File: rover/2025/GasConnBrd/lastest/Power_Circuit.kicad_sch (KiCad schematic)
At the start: 0 parts

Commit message: PCB finit
A faire approuver au besoin
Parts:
- added C18, C19, C24, C25: 10uF, Capacitor_SMD:C_0805_2012Metric_Pad1.18x1.45mm_HandSolder, symbol RoverLibrary:C_0805
- added D4: CVJ10F30, RoverFootprint:Diode_schottky-CVJ10F30, symbol RoverLibrary:Diode_Schottchy_CVJ10F30
- added J3, J6: Eth-Horiz, RoverFootprint:Ethernet_Horizontal, symbol RoverLibrary:Eth-Horiz-54601-908WPLF
- added TP6, TP7: TestPoint, TestPoint:TestPoint_Plated_Hole_D2.0mm, symbol RoverLibrary:TestPoint
- added U1: R-78E5.0-0.5, Converter_DCDC:Converter_DCDC_RECOM_R-78E-0.5_THT, symbol Regulator_Switching:R-78E5.0-0.5
- added U7: LDO-TLV74033PDBVR, Package_TO_SOT_SMD:SOT-23-5_HandSoldering, symbol RoverLibrary:LDO-TLV74033PDBVR
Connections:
- new net +24V: C19.1, J3.5, J3.7, J6.5, J6.7, U1.1 (IN)
- new net +3.3V: C24.1, TP6.1, U7.5 (OUTPUT)
- new net +5V: C18.1, D4.4, D4.5, TP7.1, U7.1 (INPUT), U7.3 (EN)
- new net +5V_ETH: C25.1, D4.3, U1.3 (OUT)
- new net +5V_USB: D4.1
- new net CAN_N: J3.2 (CANL), J6.3
- new net CAN_P: J3.1 (CANH), J6.4
- new net GND: C18.2, C19.2, C24.2, C25.2, J3.6, J3.8, J6.6, J6.8, U1.2 (GND), U7.2 (GND)
- no-connect marks 0 -> 5
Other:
- note added: "* C_in and C_out optionnal according to datasheet pads will be there if need be, but not soldered"
- note added: "5V Power Jumper"
- note added: "Data Connectors"
- note added: "ESP LDO"
- note added: "Power"
- note added: "Protection"
- note added: "Stepdown 5V"

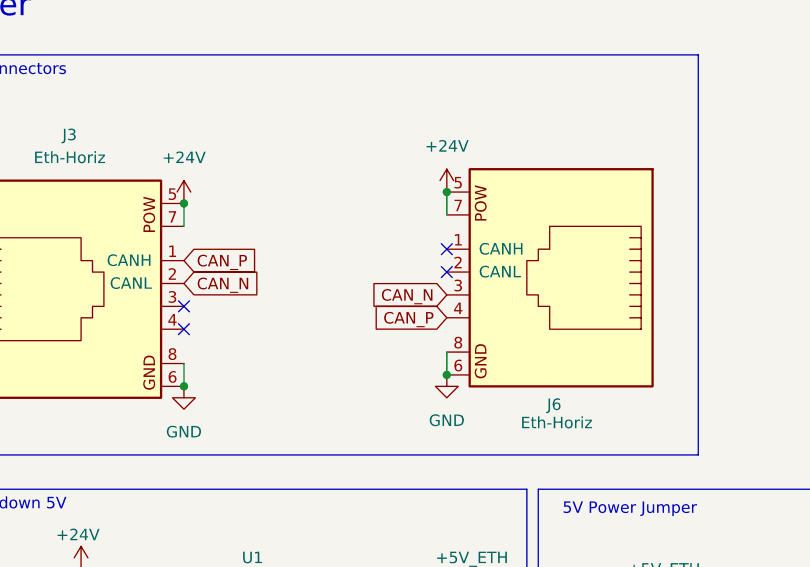
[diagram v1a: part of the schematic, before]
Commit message: PCB GAS Version 2 (compact) finit!
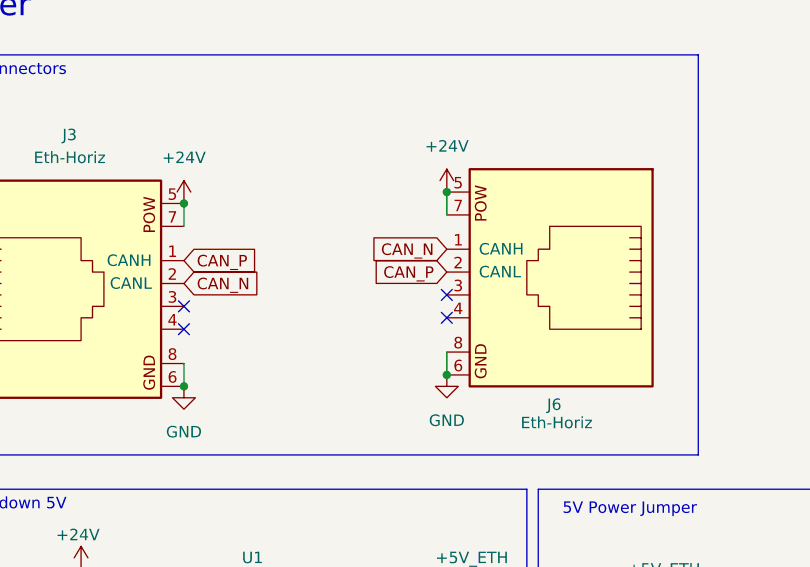
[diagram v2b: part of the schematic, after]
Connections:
- net CAN_N: now also J6.1 (CANH); no longer J6.3
- net CAN_P: now also J6.2 (CANL); no longer J6.4
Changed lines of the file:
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@@
 	)
 	(no_connect
-		(at 77.47 50.8)
-	)
-	(no_connect
-		(at 77.47 53.34)
+		(at 77.47 58.42)
 	)
 	(no_connect
 		(at 48.26 57.15)
+	)
+	(no_connect
+		(at 77.47 55.88)
 	)
 	(no_connect
@@
 	(global_label "CAN_P"
 		(shape input)
-		(at 77.47 58.42 180)
+		(at 77.47 53.34 180)
 		(fields_autoplaced yes)
 		(effects
@@
 		)
 		(property "Intersheetrefs" "${INTERSHEET_REFS}"
-			(at 68.5581 58.42 0)
+			(at 68.5581 53.34 0)
 			(effects
 				(font
@@
 	(global_label "CAN_N"
 		(shape input)
-		(at 77.47 55.88 180)
+		(at 77.47 50.8 180)
 		(fields_autoplaced yes)
 		(effects
@@
 		)
 		(property "Intersheetrefs" "${INTERSHEET_REFS}"
-			(at 68.4976 55.88 0)
+			(at 68.4976 50.8 0)
 			(effects
 				(font

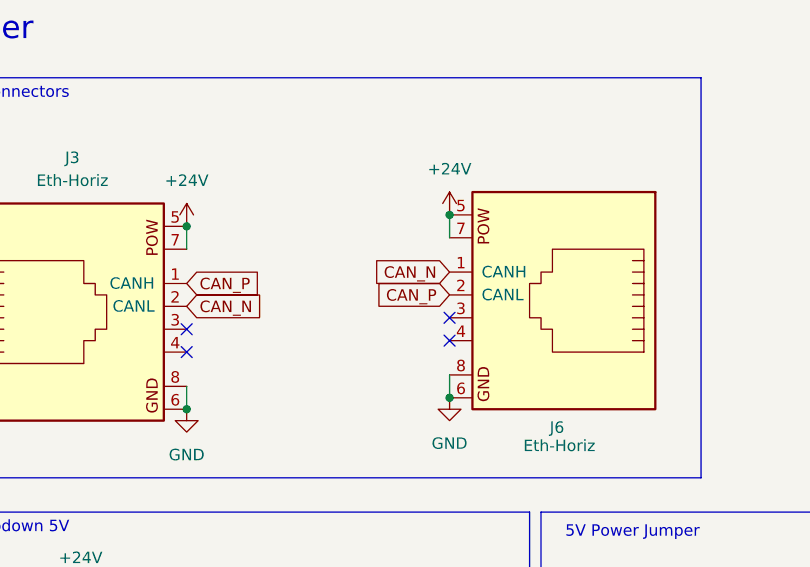
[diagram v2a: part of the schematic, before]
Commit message: PCB avec bug fixed
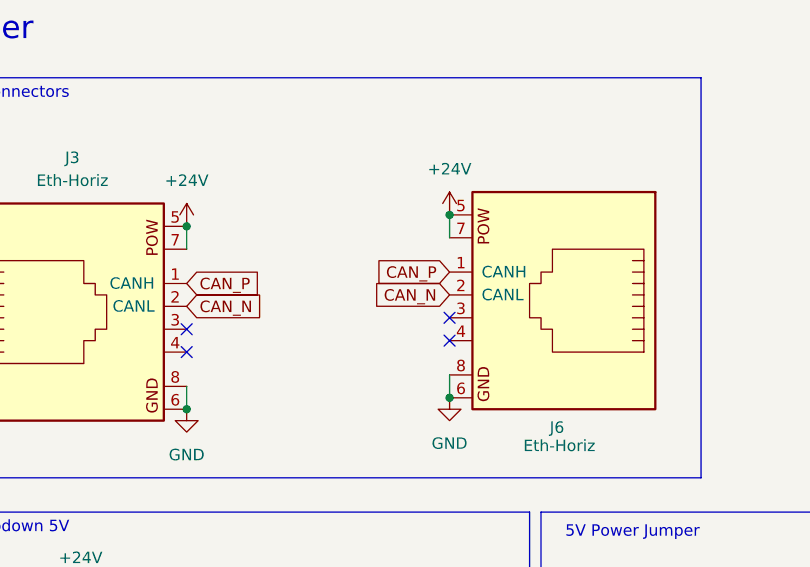
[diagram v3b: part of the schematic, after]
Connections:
- net CAN_N: now also J6.2 (CANL); no longer J6.1 (CANH)
- net CAN_P: now also J6.1 (CANH); no longer J6.2 (CANL)
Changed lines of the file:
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@@
 		)
 	)
-	(global_label "CAN_P"
+	(global_label "CAN_N"
 		(shape input)
 		(at 77.47 53.34 180)
@@
 		)
 		(property "Intersheetrefs" "${INTERSHEET_REFS}"
-			(at 68.5581 53.34 0)
+			(at 68.4976 53.34 0)
 			(effects
 				(font
@@
 		)
 	)
-	(global_label "CAN_N"
+	(global_label "CAN_P"
 		(shape input)
 		(at 77.47 50.8 180)
@@
 		)
 		(property "Intersheetrefs" "${INTERSHEET_REFS}"
-			(at 68.4976 50.8 0)
+			(at 68.5581 50.8 0)
 			(effects
 				(font
